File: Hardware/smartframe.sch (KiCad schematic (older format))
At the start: 29 parts, among them J1 USB_B, J2 Micro_SD_Card, SW1 Reset, U1 F1C100s, Y1 24MHz

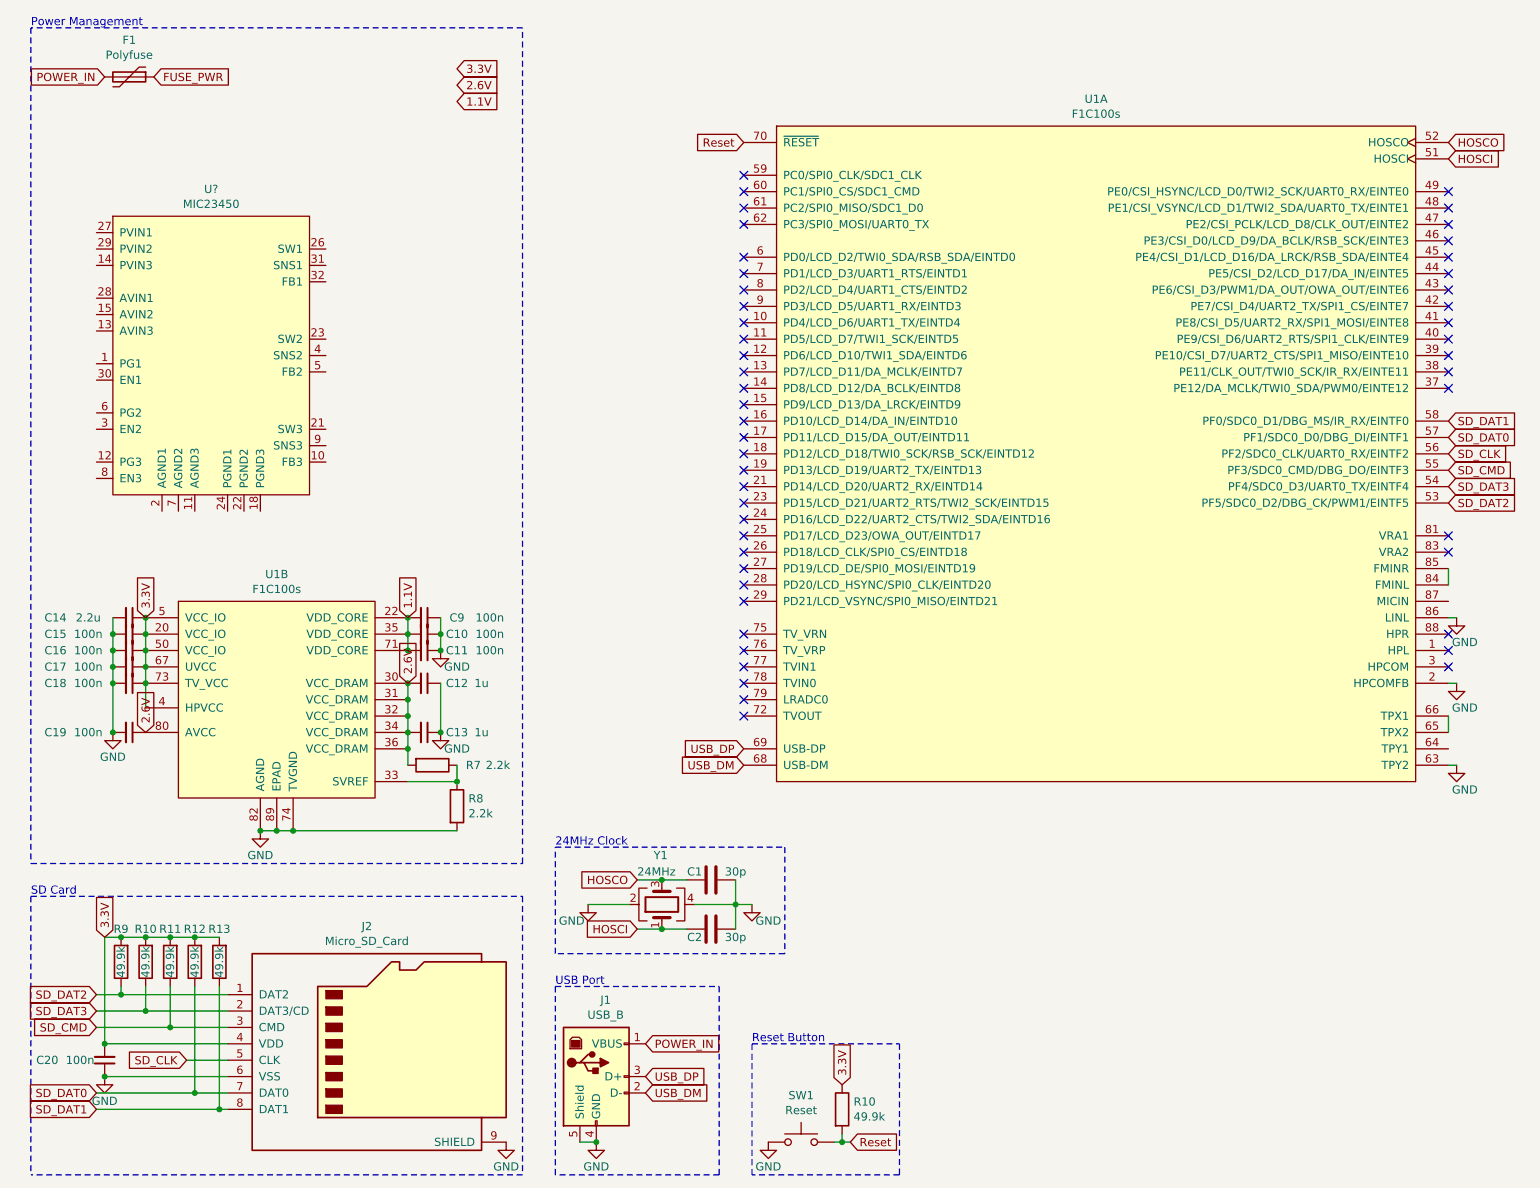
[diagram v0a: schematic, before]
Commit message: Updating power delivery
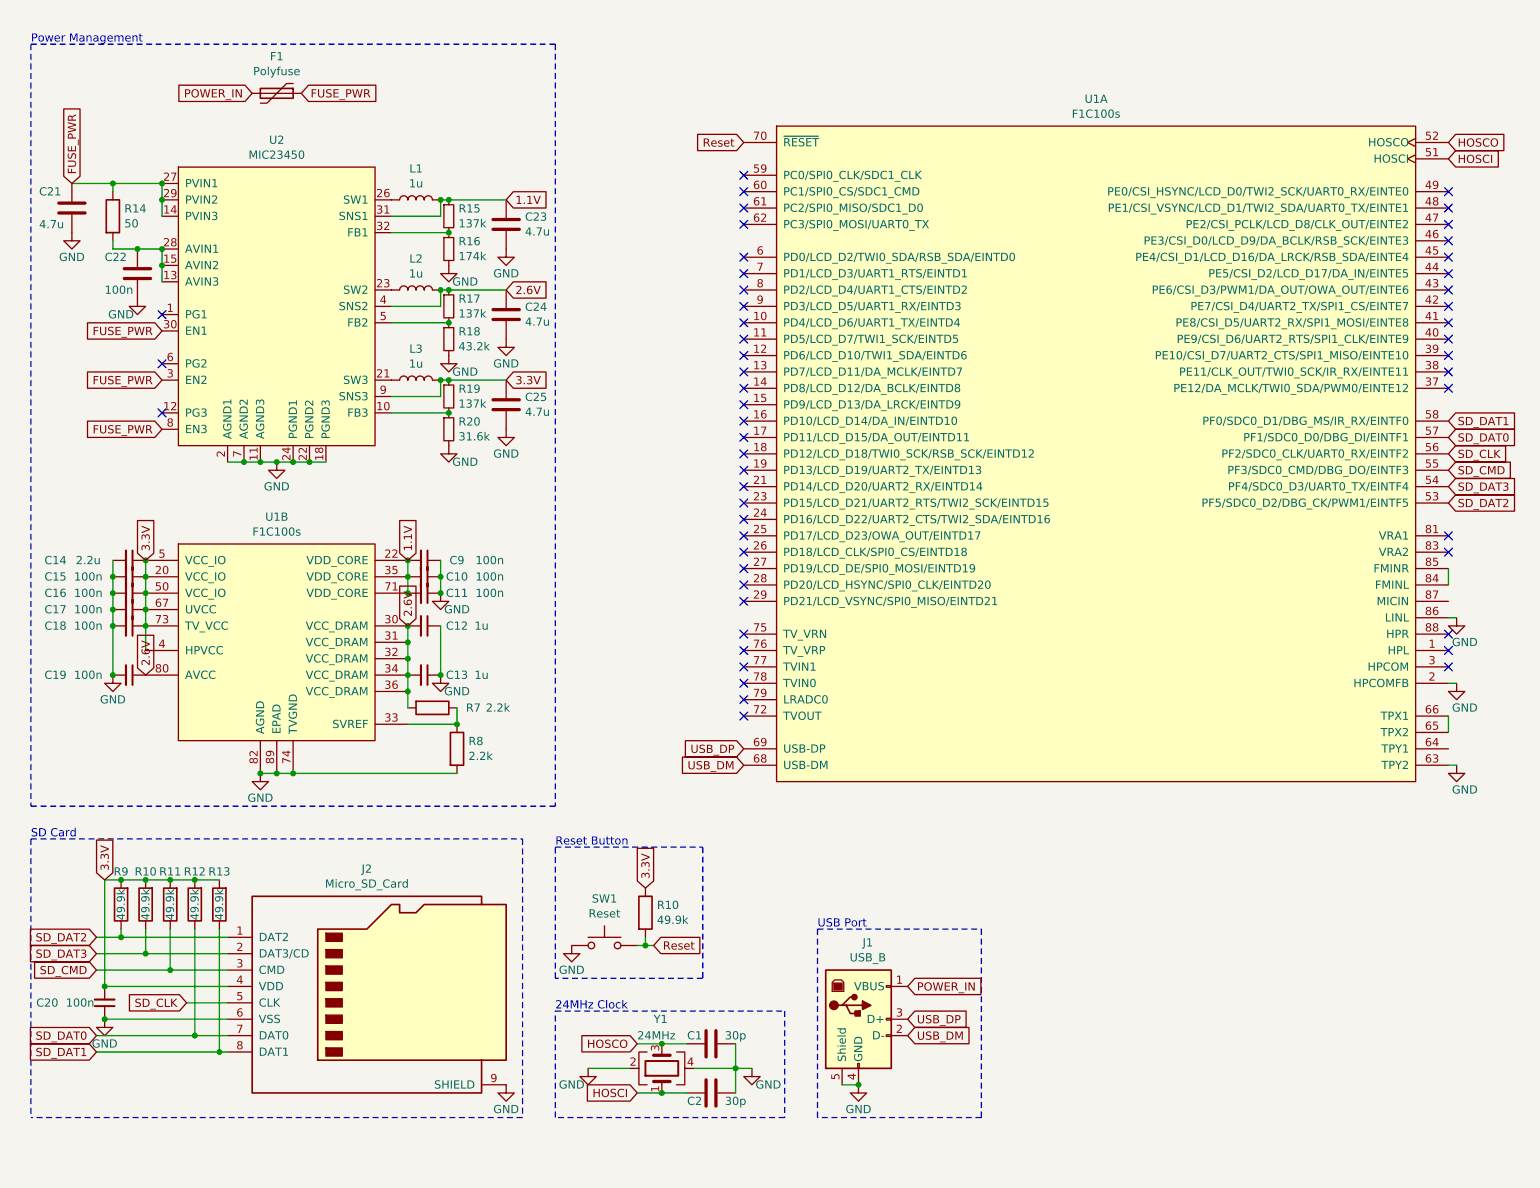
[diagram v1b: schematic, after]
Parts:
- added C21, C23, C24, C25: 4.7u, symbol Device:C
- added C22: 100n, symbol Device:C
- added L1, L2, L3: 1u, symbol Device:L
- added R14: 50, symbol Device:R
- added R15, R17, R19: 137k, symbol Device:R_Small
- added R16: 174k, symbol Device:R_Small
- added R18: 43.2k, symbol Device:R_Small
- added R20: 31.6k, symbol Device:R_Small
- gave numbers to parts that had none: 1
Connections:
- net 1.1V: now also U2.31 (SNS1), C23.1, L1.2, R15.1
- net 2.6V: now also U2.4 (SNS2), C24.1, L2.2, R17.1
- net 3.3V: now also U2.9 (SNS3), C25.1, L3.2, R19.1
- net FUSE_PWR: now also U2.14 (PVIN3), U2.27 (PVIN1), U2.29 (PVIN2), U2.3 (EN2), U2.30 (EN1), U2.8 (EN3), C21.1, R14.1
- net GND: now also U2.11 (AGND3), U2.18 (PGND3), U2.2 (AGND1), U2.22 (PGND2), U2.24 (PGND1), U2.7 (AGND2), C21.2, C22.2, C23.2, C24.2, C25.2, R16.2, R18.2, R20.2
- net at U2.10 (FB3): now also R19.2, R20.1
- net at U2.13 (AVIN3): now also U2.15 (AVIN2), U2.28 (AVIN1), C22.1, R14.2
- net at U2.21 (SW3): now also L3.1
- net at U2.23 (SW2): now also L2.1
- net at U2.26 (SW1): now also L1.1
- net at U2.32 (FB1): now also R15.2, R16.1
- net at U2.5 (FB2): now also R17.2, R18.1
- no-connect marks 50 -> 53
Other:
- moved on the sheet: C1, C10, C11, C12, C13, C14, C15, C16, C17, C18, C19, C2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
